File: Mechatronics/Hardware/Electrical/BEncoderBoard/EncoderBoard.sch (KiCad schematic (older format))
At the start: 46 parts, among them IC1 RN4020-V_RM120, IC2 TP4056, IC3 DW01+G, J1 Conn_01x07_Male, J4 Barrel_Jack_Switch, J5 Batt+, J7 Batt-, Q1 FS8205, Q2 Q_PMOS_GSD, U1 STM32F103C8T6, U2 ITR1802A, U3 ITR1802B, U5 SSD1306OLED, U6 LTC2430, Y1 8Mhz

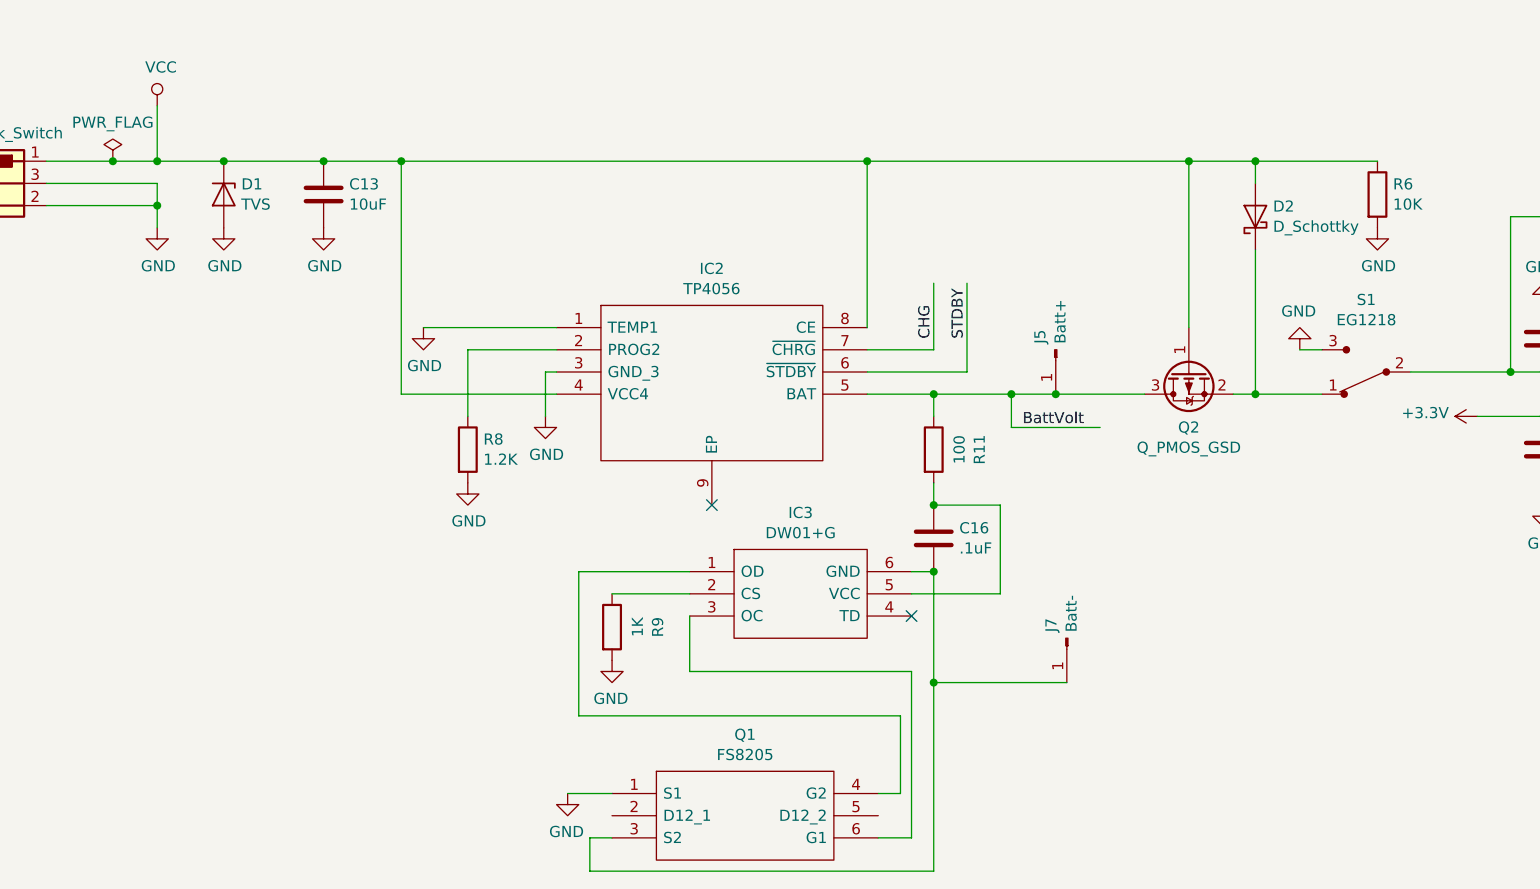
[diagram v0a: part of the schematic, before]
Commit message: Added changes
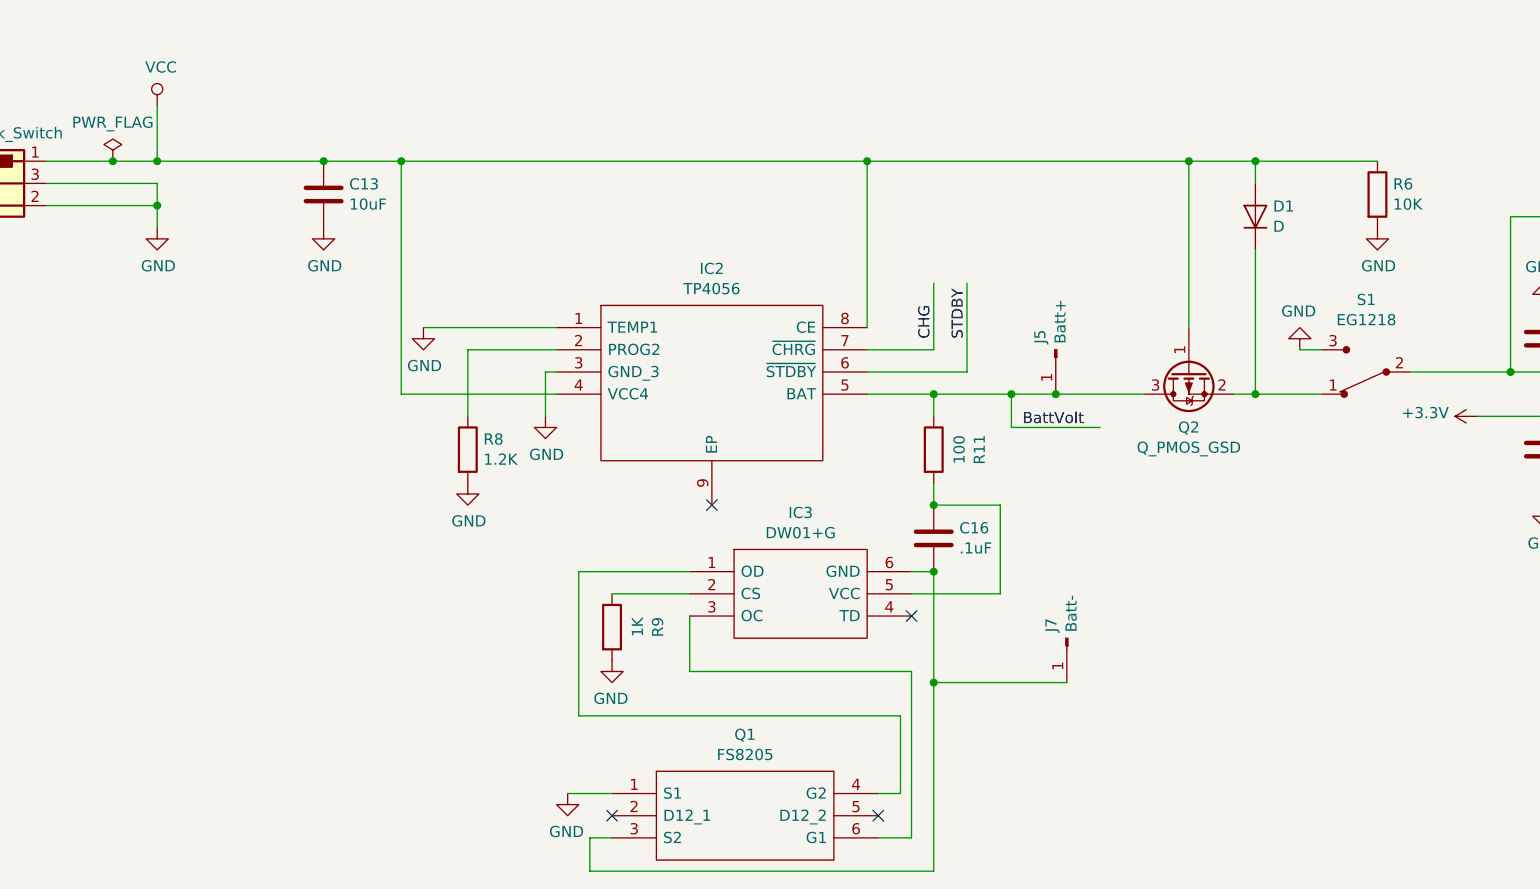
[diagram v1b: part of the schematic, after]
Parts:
- removed D1: TVS, Encoder:D_DO-201AD_P15.24mm_Horizontal, symbol Device:D_Zener
- removed D2: D_Schottky, Encoder:D_DO-201AD_P15.24mm_Horizontal, symbol Device:D_Schottky
- added D1: D, Encoder:D_SMA, symbol Device:D
- J5, J7: footprint Encoder:PinHeader_1x01_P2.54mm_Vertical -> Encoder:No3dmodelPinHeader_1x01_P2.54mm_Vertical
- Q2: footprint (none) -> Encoder:SOT-23
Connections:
- wire segments 168 -> 167
- no-connect marks 34 -> 36
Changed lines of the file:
@@
 Wire Wire Line
 	5650 6750 5650 6900
-$Comp
-L Device:D_Zener D1
-U 1 1 5D40B7CD
-P 2100 5850
-F 0 "D1" V 2054 5929 50  0000 L CNN
-F 1 "TVS" V 2145 5929 50  0000 L CNN
-F 2 "Encoder:D_DO-201AD_P15.24mm_Horizontal" H 2100 5850 50  0001 C CNN
-F 3 "~" H 2100 5850 50  0001 C CNN
-	1    2100 5850
-	0    1    1    0
-$EndComp
 Connection ~ 6450 5700
 Wire Wire Line
@@
 $EndComp
 $Comp
-L Device:D_Schottky D2
-U 1 1 5D40B8AB
-P 6750 5950
-F 0 "D2" V 6796 5871 50  0000 R CNN
-F 1 "D_Schottky" V 6705 5871 50  0000 R CNN
-F 2 "Encoder:D_DO-201AD_P15.24mm_Horizontal" H 6750 5950 50  0001 C CNN
-F 3 "~" H 6750 5950 50  0001 C CNN
-	1    6750 5950
-	0    -1   -1   0
-$EndComp
-$Comp
 L Encoder:LTC2430 U6
 U 1 1 5D41A14E
@@
 Wire Wire Line
 	6750 5700 7300 5700
-Wire Wire Line
-	6750 6100 6750 6750
 Wire Wire Line
 	7900 6650 7900 5950
@@
 F 0 "J7" H 5873 7780 50  0000 R CNN
 F 1 "Batt-" H 5873 7871 50  0000 R CNN
-F 2 "Encoder:PinHeader_1x01_P2.54mm_Vertical" H 5900 7850 50  0001 C CNN
+F 2 "Encoder:No3dmodelPinHeader_1x01_P2.54mm_Vertical" H 5900 7850 50  0001 C CNN
 F 3 "~" H 5900 7850 50  0001 C CNN
 	1    5900 7850
@@
 F 0 "J5" H 5823 6480 50  0000 R CNN
 F 1 "Batt+" H 5823 6571 50  0000 R CNN
-F 2 "Encoder:PinHeader_1x01_P2.54mm_Vertical" H 5850 6550 50  0001 C CNN
+F 2 "Encoder:No3dmodelPinHeader_1x01_P2.54mm_Vertical" H 5850 6550 50  0001 C CNN
 F 3 "~" H 5850 6550 50  0001 C CNN
 	1    5850 6550
@@
 Wire Wire Line
 	1800 5450 1800 5700
-Wire Wire Line
-	1800 5700 2100 5700
-Connection ~ 2100 5700
-$Comp
-L power:GND #PWR06
-U 1 1 5D706B3B
-P 2100 6000
-F 0 "#PWR06" H 2100 5750 50  0001 C CNN
-F 1 "GND" H 2105 5827 50  0000 C CNN
-F 2 "" H 2100 6000 50  0001 C CNN
-F 3 "" H 2100 6000 50  0001 C CNN
-	1    2100 6000
-	1    0    0    -1
-$EndComp
 Connection ~ 1800 5700
 $Comp
@@
 Wire Wire Line
 	1700 900  2150 900
-Wire Wire Line
-	2100 5700 2550 5700
 Wire Wire Line
 	5000 5700 6450 5700
@@
 F 0 "Q2" H 6450 6500 50  0000 C CNN
 F 1 "Q_PMOS_GSD" H 6450 6409 50  0000 C CNN
-F 2 "" V 6650 6550 50  0001 C CNN
+F 2 "Encoder:SOT-23" V 6650 6550 50  0001 C CNN
 F 3 "~" V 6450 6750 50  0001 C CNN
 	1    6450 6700
 	1    0    0    -1
 $EndComp
+Wire Wire Line
+	1800 5700 2550 5700
+$Comp
+L Device:D D1
+U 1 1 5D4F6601
+P 6750 5950
+F 0 "D1" V 6796 5871 50  0000 R CNN
+F 1 "D" V 6705 5871 50  0000 R CNN
+F 2 "Encoder:D_SMA" H 6750 5950 50  0001 C CNN
+F 3 "~" H 6750 5950 50  0001 C CNN
+	1    6750 5950
+	0    -1   -1   0
+$EndComp
+Wire Wire Line
+	6750 6100 6750 6750
+NoConn ~ 3850 8650
+NoConn ~ 5050 8650
 $EndSCHEMATC
